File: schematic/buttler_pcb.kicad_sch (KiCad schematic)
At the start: 24 parts, among them J1 HL, J2 HR, J3 ISP, J4 RF Receiver, J5 IO, J6 ISP 2, SW1 Reset, SW2 Pgm/Factory, U1 PC817, U2 PC817, U3 PC817

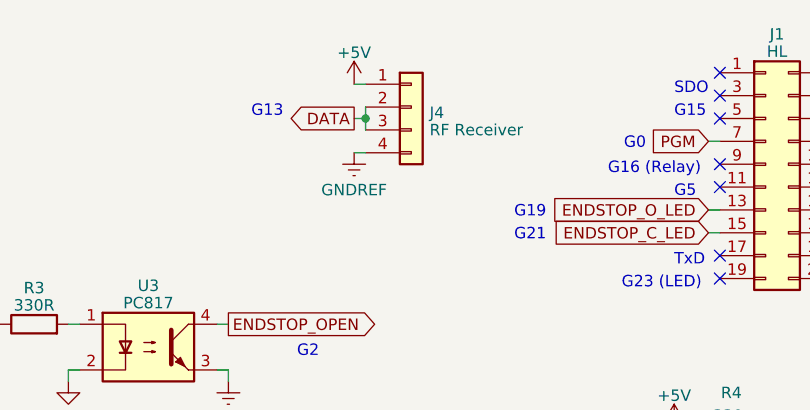
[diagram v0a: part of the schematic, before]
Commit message: Repo Sync
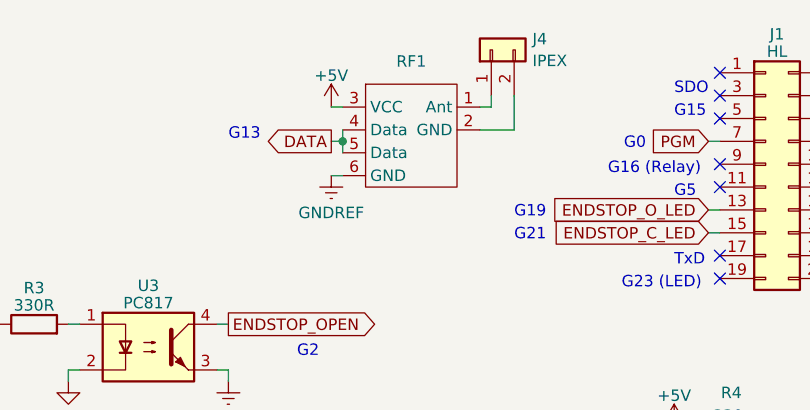
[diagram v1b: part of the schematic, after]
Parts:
- removed J4: RF Receiver, Connector_PinHeader_2.54mm:PinHeader_1x04_P2.54mm_Vertical, symbol Connector_Generic:Conn_01x04
- added J4: IPEX, buttler:IPEX_20279-001E-03, symbol Connector_Generic:Conn_01x02
- added RF1: ~, buttler:RXB12, symbol buttler:RXB12
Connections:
- net +5V: now also RF1.3 (VCC)
- net DATA: now also RF1.4 (Data), RF1.5 (Data)
- net GNDREF: now also RF1.6 (GND)
- new net: J4.1 (Pin_1), RF1.1 (Ant)
- new net: J4.2 (Pin_2), RF1.2 (GND)
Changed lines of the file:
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@@
 	)
 	(junction
-		(at 143.51 29.21)
-		(diameter 0)
-		(color 0 0 0 0)
-	)
-	(junction
 		(at 226.06 106.68)
 		(diameter 0)
@@
 	)
 	(junction
+		(at 140.97 31.75)
+		(diameter 0)
+		(color 0 0 0 0)
+	)
+	(junction
 		(at 177.8 77.47)
 		(diameter 0)
@@
 	(wire
 		(pts
-			(xy 142.24 33.02) (xy 143.51 33.02)
+			(xy 139.7 35.56) (xy 140.97 35.56)
 		)
 		(stroke
@@
 	(wire
 		(pts
-			(xy 143.51 29.21) (xy 143.51 30.48)
+			(xy 157.48 27.94) (xy 156.21 27.94)
+		)
+		(stroke
+			(width 0)
+			(type default)
+		)
+	)
+	(wire
+		(pts
+			(xy 140.97 31.75) (xy 140.97 33.02)
 		)
 		(stroke
@@
 	(wire
 		(pts
-			(xy 142.24 29.21) (xy 143.51 29.21)
+			(xy 139.7 31.75) (xy 140.97 31.75)
 		)
 		(stroke
@@
 	(wire
 		(pts
+			(xy 160.02 26.67) (xy 160.02 30.48)
+		)
+		(stroke
+			(width 0)
+			(type default)
+		)
+	)
+	(wire
+		(pts
 			(xy 128.27 90.17) (xy 127 90.17)
 		)
@@
 	(wire
 		(pts
-			(xy 142.24 25.4) (xy 143.51 25.4)
+			(xy 139.7 27.94) (xy 140.97 27.94)
 		)
 		(stroke
@@
 	(wire
 		(pts
+			(xy 160.02 30.48) (xy 156.21 30.48)
+		)
+		(stroke
+			(width 0)
+			(type default)
+		)
+	)
+	(wire
+		(pts
 			(xy 88.9 73.66) (xy 90.17 73.66)
 		)
@@
 	(wire
 		(pts
-			(xy 143.51 27.94) (xy 143.51 29.21)
+			(xy 140.97 30.48) (xy 140.97 31.75)
 		)
 		(stroke
@@
 		)
 	)
+	(wire
+		(pts
+			(xy 157.48 26.67) (xy 157.48 27.94)
+		)
+		(stroke
+			(width 0)
+			(type default)
+		)
+	)
 	(text "G17"
 		(exclude_from_sim no)
@@
 	(text "G13"
 		(exclude_from_sim no)
-		(at 130.81 29.21 0)
+		(at 128.27 31.75 0)
 		(effects
 			(font
@@
 	(global_label "DATA"
 		(shape output)
-		(at 142.24 29.21 180)
+		(at 139.7 31.75 180)
 		(fields_autoplaced yes)
 		(effects
@@
 		)
 		(property "Intersheetrefs" "${INTERSHEET_REFS}"
-			(at 134.9194 29.21 0)
+			(at 132.3794 31.75 0)
 			(effects
 				(font
@@
 	(symbol
 		(lib_id "power:+5V")
-		(at 142.24 25.4 0)
+		(at 139.7 27.94 0)
 		(unit 1)
 		(exclude_from_sim no)
@@
 		(fields_autoplaced yes)
 		(property "Reference" "#PWR09"
-			(at 142.24 29.21 0)
+			(at 139.7 31.75 0)
 			(effects
 				(font
@@
 		)
 		(property "Value" "+5V"
-			(at 142.24 21.8981 0)
+			(at 139.7 24.4381 0)
 			(effects
 				(font
@@
 		)
 		(property "Footprint" ""
-			(at 142.24 25.4 0)
+			(at 139.7 27.94 0)
 			(effects
 				(font
@@
 		)
 		(property "Datasheet" ""
-			(at 142.24 25.4 0)
+			(at 139.7 27.94 0)
 			(effects
 				(font
@@
 		)
 		(property "Description" ""
-			(at 142.24 25.4 0)
+			(at 139.7 27.94 0)
 			(effects
 				(font
@@
 	)
 	(symbol
+		(lib_id "buttler:RXB12")
+		(at 148.59 31.75 0)
+		(unit 1)
+		(exclude_from_sim no)
+		(in_bom yes)
+		(on_board yes)
+		(dnp no)
+		(fields_autoplaced yes)
+		(property "Reference" "RF1"
+			(at 148.59 22.8685 0)
+			(effects
+				(font
+					(size 1.27 1.27)
+				)
+			)
+		)
+		(property "Value" "~"
+			(at 148.59 24.5499 0)
+			(effects
+				(font
+					(size 1.27 1.27)
+				)
+			)
+		)
+		(property "Footprint" "buttler:RXB12"
+			(at 148.59 31.75 0)
+			(effects
+				(font
+					(size 1.27 1.27)
+				)
+				(hide yes)
+			)
+		)
+		(property "Datasheet" ""
+			(at 148.59 31.75 0)
+			(effects
+				(font
+					(size 1.27 1.27)
+				)
+				(hide yes)
+			)
+		)
+		(property "Description" ""
+			(at 148.59 31.75 0)
+			(effects
+				(font
+					(size 1.27 1.27)
+				)
+				(hide yes)
+			)
+		)
+		(pin "3"
+		)
+		(pin "1"
+		)
+		(pin "6"
+		)
+		(pin "2"
+		)
+		(pin "4"
+		)
+		(pin "5"
+		)
+		(instances
+			(project ""
+				(path "/caf301de-9bdf-4647-9950-327c7a304977"
+					(reference "RF1")
+					(unit 1)
+				)
+			)
+		)
+	)
+	(symbol
 		(lib_id "power:GNDREF")
 		(at 128.27 74.93 0)
@@
 	)
 	(symbol
+		(lib_id "Connector_Generic:Conn_01x02")
+		(at 157.48 21.59 90)
+		(unit 1)
+		(exclude_from_sim no)
+		(in_bom yes)
+		(on_board yes)
+		(dnp no)
+		(fields_autoplaced yes)
+		(property "Reference" "J4"
+			(at 162.052 20.3778 90)
+			(effects
+				(font
+					(size 1.27 1.27)
+				)
+				(justify right)
+			)
+		)
+		(property "Value" "IPEX"
+			(at 162.052 22.8021 90)
+			(effects
+				(font
+					(size 1.27 1.27)
+				)
+				(justify right)
+			)
+		)
+		(property "Footprint" "buttler:IPEX_20279-001E-03"
+			(at 157.48 21.59 0)
+			(effects
+				(font
+					(size 1.27 1.27)
+				)
+				(hide yes)
+			)
+		)
+		(property "Datasheet" "~"
+			(at 157.48 21.59 0)
+			(effects
+				(font
+					(size 1.27 1.27)
+				)
+				(hide yes)
+			)
+		)
+		(property "Description" "Generic connector, single row, 01x02, script generated (kicad-library-utils/schlib/autogen/connector/)"
+			(at 157.48 21.59 0)
+			(effects
+				(font
+					(size 1.27 1.27)
+				)
+				(hide yes)
+			)
+		)
+		(pin "2"
+		)
+		(pin "1"
+		)
+		(instances
+			(project ""
+				(path "/caf301de-9bdf-4647-9950-327c7a304977"
+					(reference "J4")
+					(unit 1)
+				)
+			)
+		)
+	)
+	(symbol
 		(lib_id "power:GNDREF")
 		(at 128.27 91.44 0)
@@
 	)
 	(symbol
-		(lib_id "Connector_Generic:Conn_01x04")
-		(at 148.59 27.94 0)
-		(unit 1)
-		(exclude_from_sim no)
-		(in_bom yes)
-		(on_board yes)
-		(dnp no)
-		(fields_autoplaced yes)
-		(property "Reference" "J4"
-			(at 150.622 28.5663 0)
-			(effects
-				(font
-					(size 1.27 1.27)
-				)
-				(justify left)
-			)
-		)
-		(property "Value" "RF Receiver"
-			(at 150.622 30.4873 0)
-			(effects
-				(font
-					(size 1.27 1.27)
-				)
-				(justify left)
-			)
-		)
-		(property "Footprint" "Connector_PinHeader_2.54mm:PinHeader_1x04_P2.54mm_Vertical"
-			(at 148.59 27.94 0)
-			(effects
-				(font
-					(size 1.27 1.27)
-				)
-				(hide yes)
-			)
-		)
-		(property "Datasheet" "~"
-			(at 148.59 27.94 0)
-			(effects
-				(font
-					(size 1.27 1.27)
-				)
-				(hide yes)
-			)
-		)
-		(property "Description" ""
-			(at 148.59 27.94 0)
-			(effects
-				(font
-					(size 1.27 1.27)
-				)
-				(hide yes)
-			)
-		)
-		(pin "1"
-		)
-		(pin "2"
-		)
-		(pin "3"
-		)
-		(pin "4"
-		)
-		(instances
-			(project "buttler_pcb"
-				(path "/caf301de-9bdf-4647-9950-327c7a304977"
-					(reference "J4")
-					(unit 1)
-				)
-			)
-		)
-	)
-	(symbol
 		(lib_id "power:GND")
 		(at 110.49 91.44 0)
@@
 	(symbol
 		(lib_id "power:GNDREF")
-		(at 142.24 33.02 0)
+		(at 139.7 35.56 0)
 		(unit 1)
 		(exclude_from_sim no)
@@
 		(fields_autoplaced yes)
 		(property "Reference" "#PWR010"
-			(at 142.24 39.37 0)
+			(at 139.7 41.91 0)
 			(effects
 				(font
@@
 		)
 		(property "Value" "GNDREF"
-			(at 142.24 37.1555 0)
+			(at 139.7 39.6955 0)
 			(effects
 				(font
@@
 		)
 		(property "Footprint" ""
-			(at 142.24 33.02 0)
+			(at 139.7 35.56 0)
 			(effects
 				(font
@@
 		)
 		(property "Datasheet" ""
-			(at 142.24 33.02 0)
+			(at 139.7 35.56 0)
 			(effects
 				(font
@@
 		)
 		(property "Description" ""
-			(at 142.24 33.02 0)
+			(at 139.7 35.56 0)
 			(effects
 				(font
